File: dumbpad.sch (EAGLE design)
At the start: 37 parts

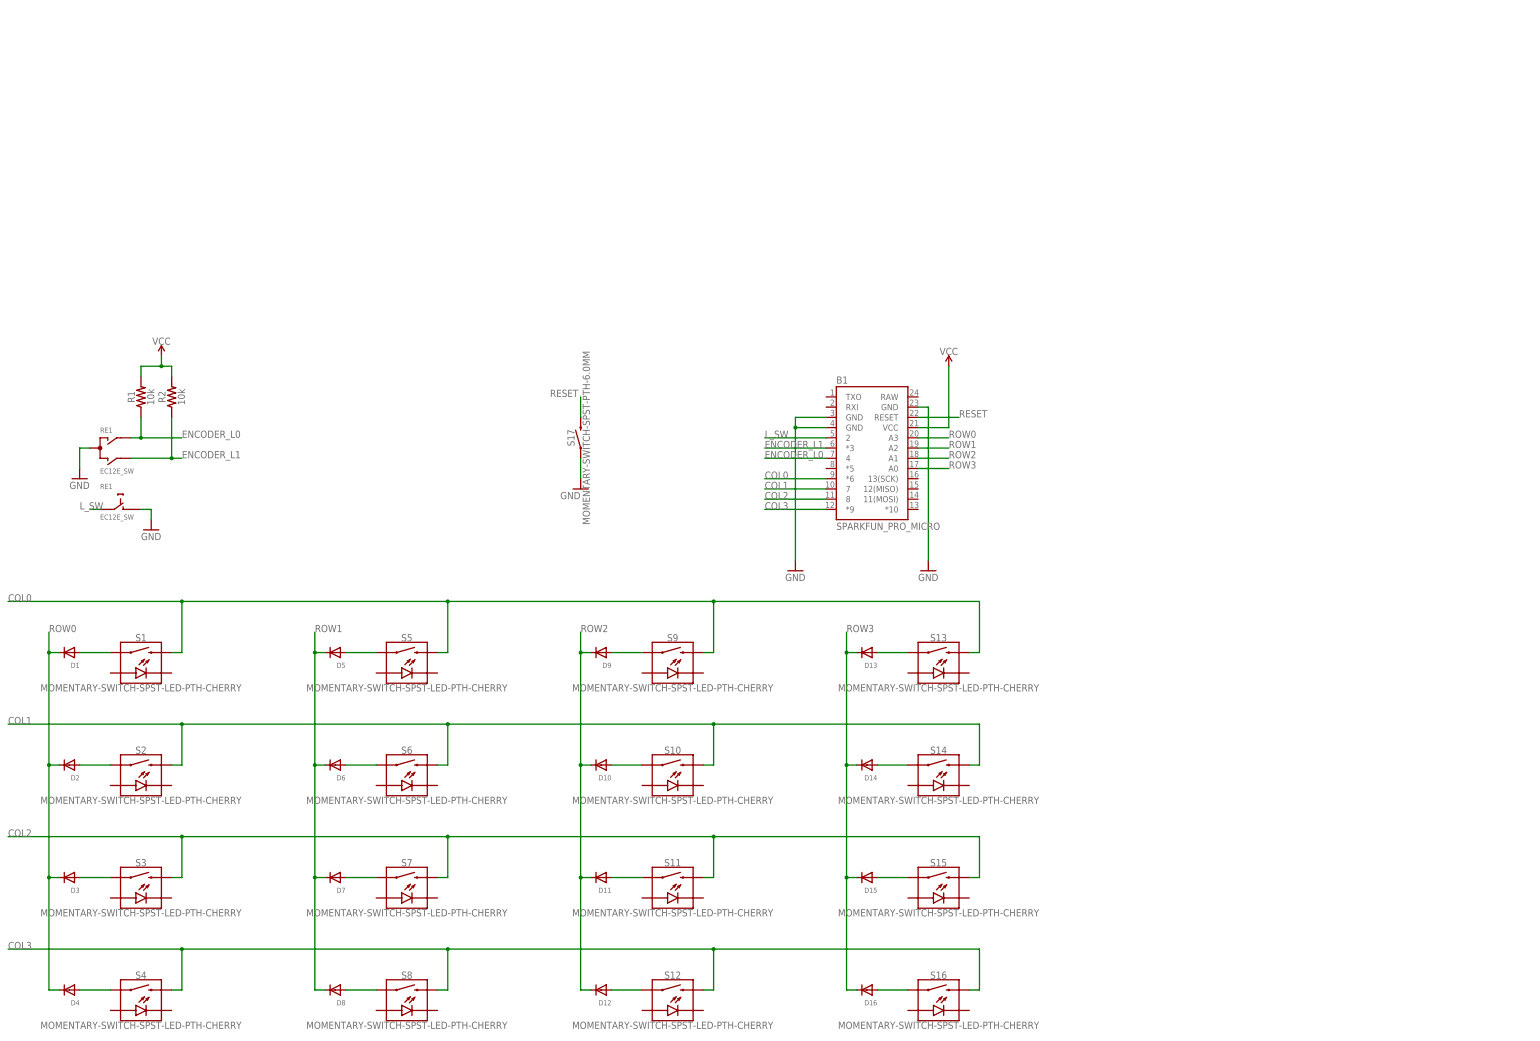
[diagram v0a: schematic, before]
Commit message: minor tweaks, sch as png
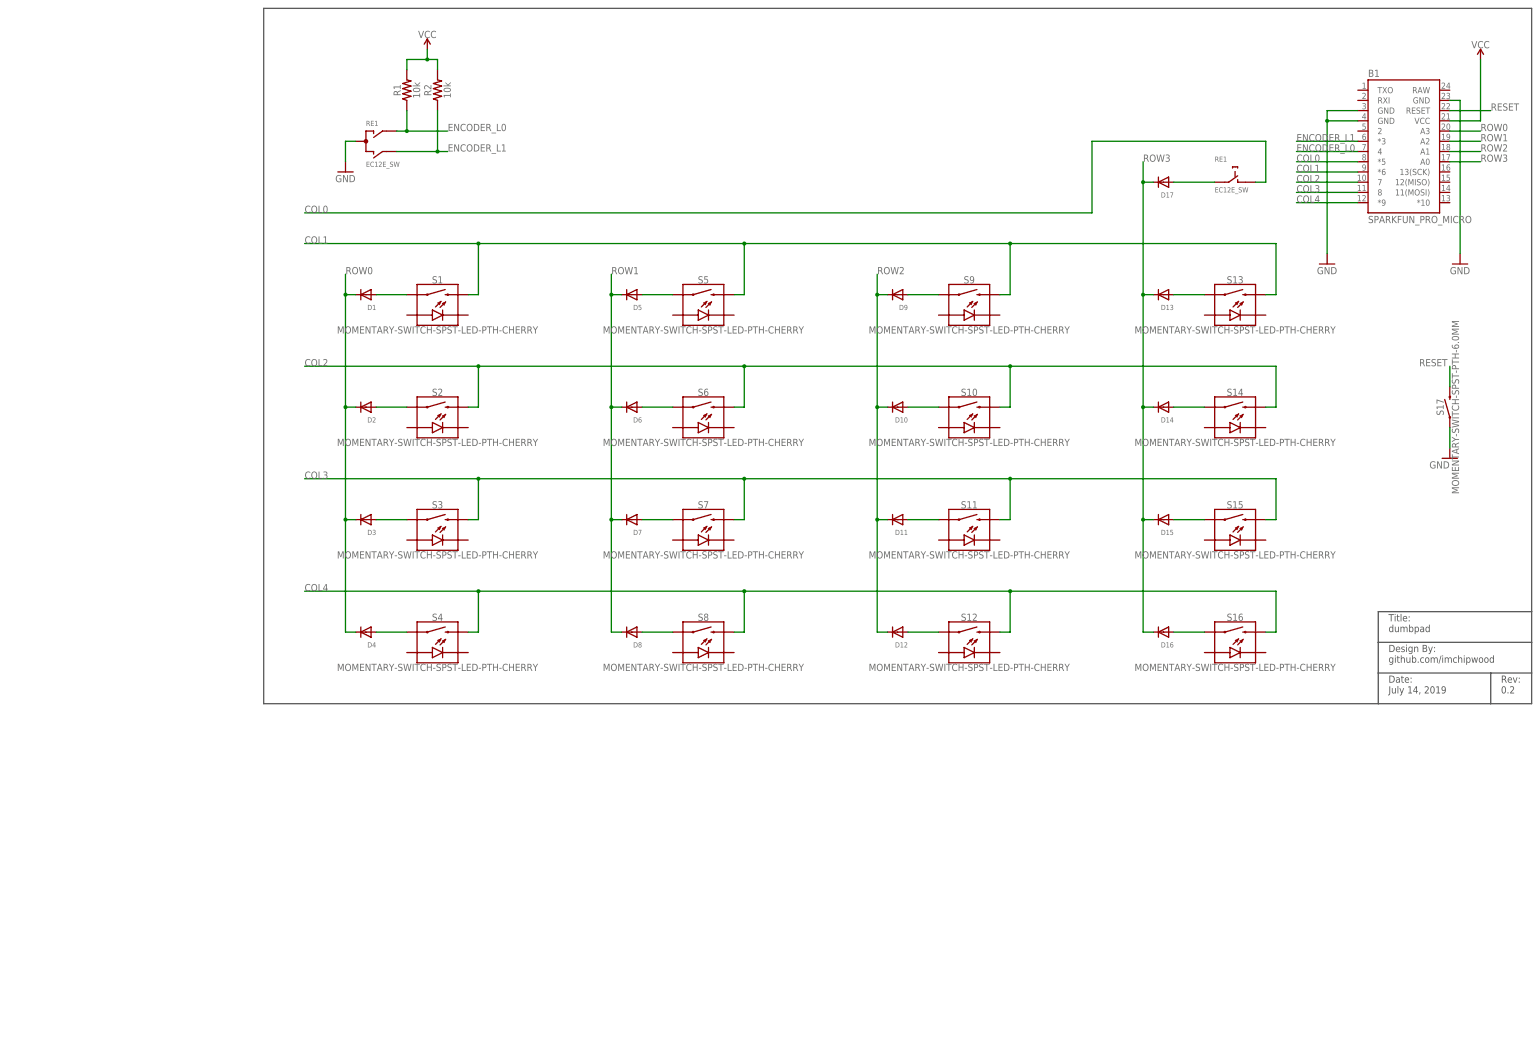
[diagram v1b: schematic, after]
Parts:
- added D17: (no value), adafruit:DIODEDO-1N4148
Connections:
- removed net L_SW: B1.2, RE1G$2.2
- new net COL4: B1.*9, S12.2, S16.2, S4.2, S8.2
- new net N$10: D17.A, RE1G$2.2
- net COL0: now also B1.*5, RE1G$2.1; no longer B1.*6, S1.2, S13.2, S5.2, S9.2
- net COL1: now also B1.*6, S1.2, S13.2, S5.2, S9.2; no longer B1.7, S10.2, S14.2, S2.2, S6.2
- net COL2: now also B1.7, S10.2, S14.2, S2.2, S6.2; no longer B1.8, S11.2, S15.2, S3.2, S7.2
- net COL3: now also B1.8, S11.2, S15.2, S3.2, S7.2; no longer B1.*9, S12.2, S16.2, S4.2, S8.2
- net GND: no longer RE1G$2.1
- net ROW3: now also D17.C
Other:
- note added: "Date: July 14, 2019"
- note added: "Design By: github.com/imchipwood"
- note added: "Rev: 0.2"
- note added: "Title: dumbpad"
- moved on the sheet: B1, D1, D10, D11, D12, D13, D14, D15, D16, D2, D3, D4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
